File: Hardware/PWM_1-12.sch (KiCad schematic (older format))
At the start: 0 parts

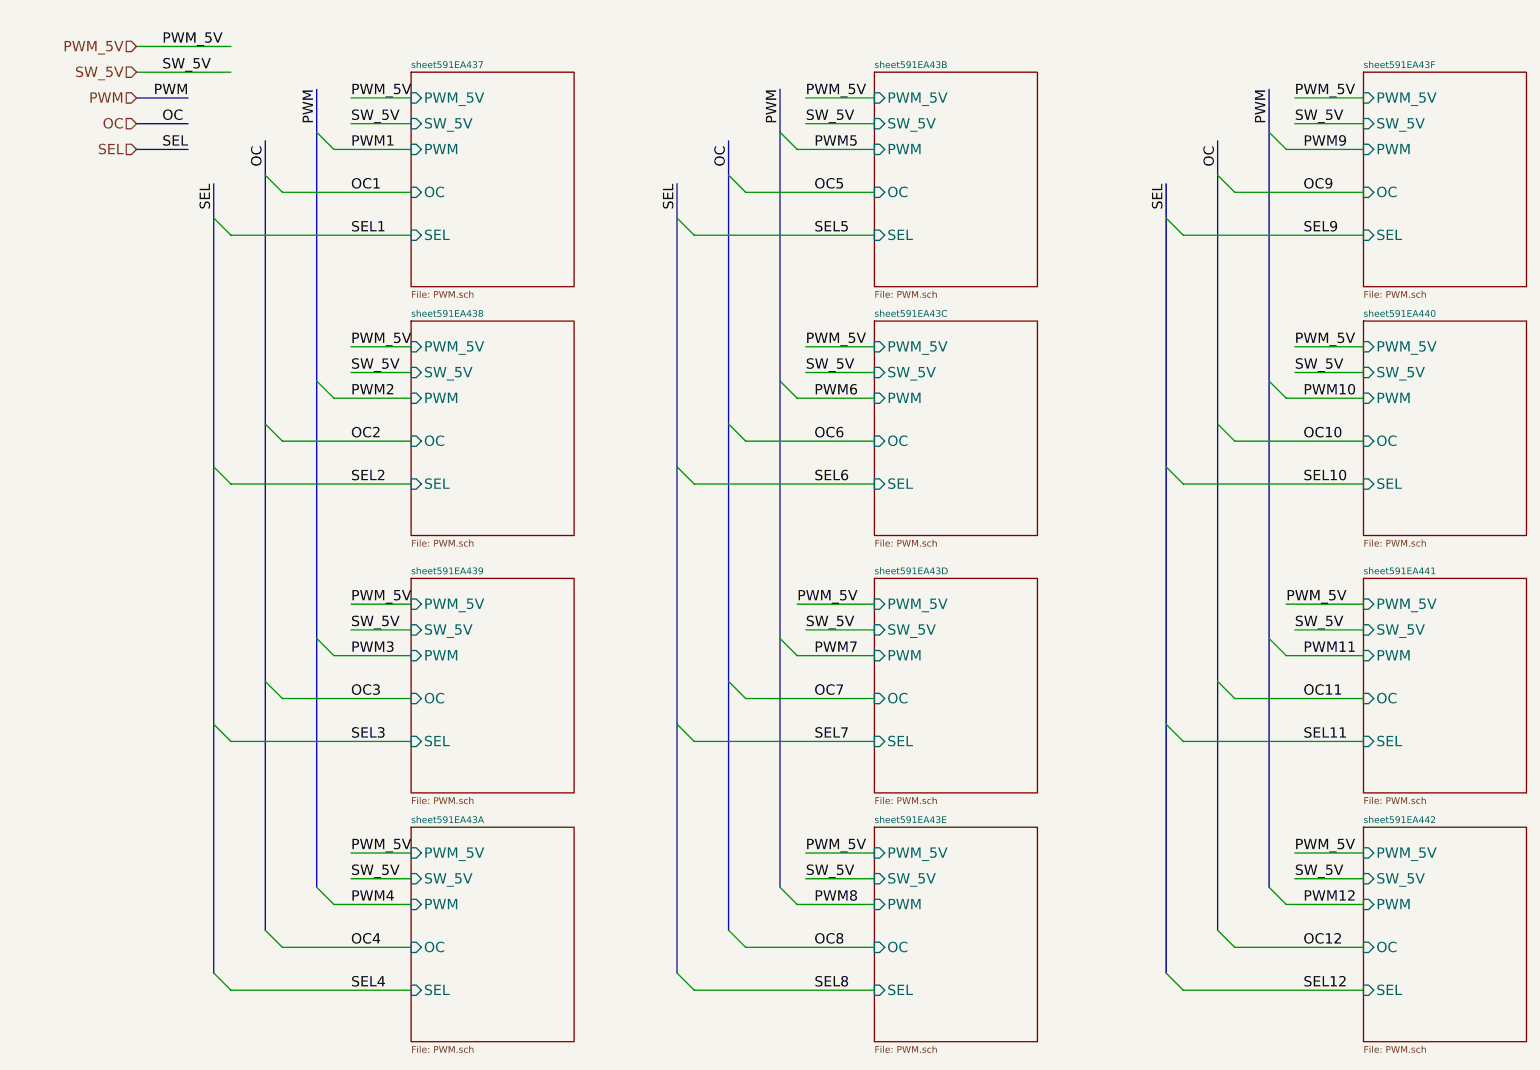
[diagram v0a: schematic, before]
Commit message: Added F7 Circuitry
Added way too much for 1 commit.
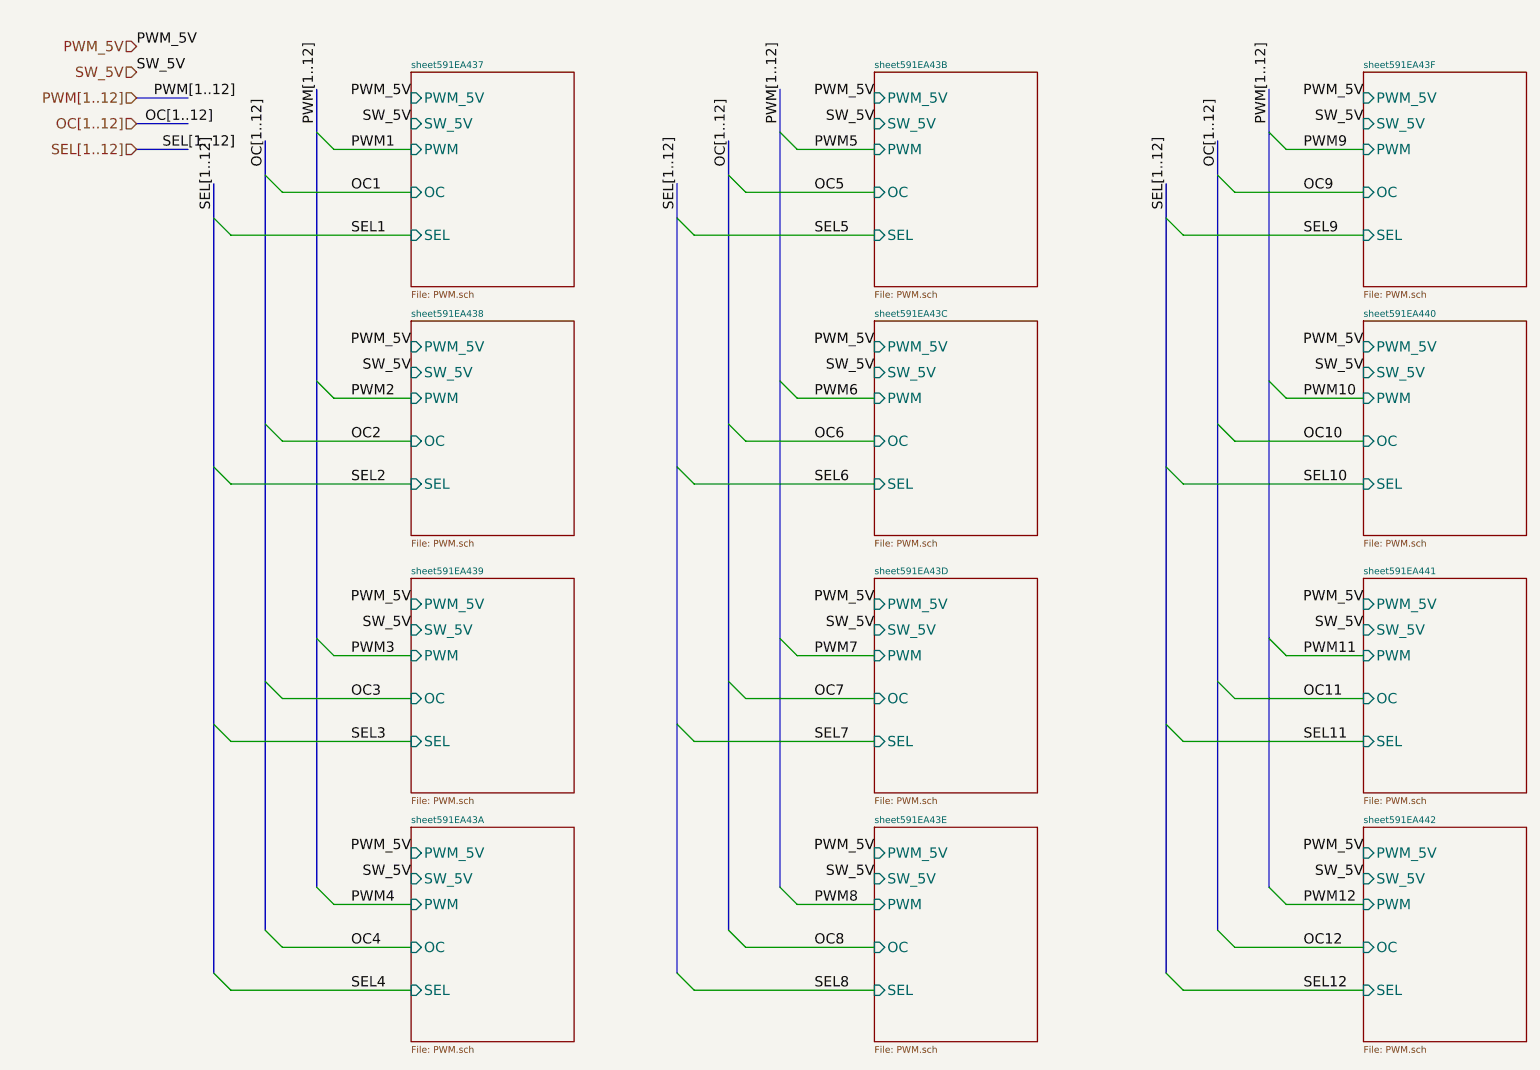
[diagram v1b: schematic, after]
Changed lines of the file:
@@
 LIBS:contrib
 LIBS:valves
+LIBS:ZeroPilot-cache
 EELAYER 25 0
 EELAYER END
 $Descr A4 11693 8268
 encoding utf-8
-Sheet 2 18
+Sheet 2 17
 Title "PWM 1-12"
 Date "2017-05-13"
@@
 PWM4
 Text Label 2150 1100 1    60   ~ 0
-PWM
+PWM[1..12]
 Entry Wire Line
 	1850 5800 1950 5900
@@
 	1850 1400 1950 1500
 Text Label 1850 1350 1    60   ~ 0
-OC
+OC[1..12]
 Entry Wire Line
 	1550 6050 1650 6150
@@
 	1550 1650 1650 1750
 Text Label 1550 1600 1    60   ~ 0
-SEL
+SEL[1..12]
 Text Label 2350 1500 0    60   ~ 0
 OC1
@@
 PWM8
 Text Label 4850 1100 1    60   ~ 0
-PWM
+PWM[1..12]
 Entry Wire Line
 	4550 5800 4650 5900
@@
 	4550 1400 4650 1500
 Text Label 4550 1350 1    60   ~ 0
-OC
+OC[1..12]
 Entry Wire Line
 	4250 6050 4350 6150
@@
 	4250 1650 4350 1750
 Text Label 4250 1600 1    60   ~ 0
-SEL
+SEL[1..12]
 Text Label 5050 1500 0    60   ~ 0
 OC5
@@
 PWM12
 Text Label 7700 1100 1    60   ~ 0
-PWM
+PWM[1..12]
 Entry Wire Line
 	7400 5800 7500 5900
@@
 	7400 1400 7500 1500
 Text Label 7400 1350 1    60   ~ 0
-OC
+OC[1..12]
 Entry Wire Line
 	7100 6050 7200 6150
@@
 	7100 1650 7200 1750
 Text Label 7100 1600 1    60   ~ 0
-SEL
+SEL[1..12]
 Text Label 7900 1500 0    60   ~ 0
 OC9
@@
 Text Label 7900 6150 0    60   ~ 0
 SEL12
-Wire Wire Line
-	2700 950  2350 950
-Wire Wire Line
-	1100 650  1650 650
-Wire Wire Line
-	2350 5350 2700 5350
-Wire Wire Line
-	5400 950  5000 950
-Wire Wire Line
-	5000 5350 5400 5350
-Wire Wire Line
-	5400 3900 4950 3900
-Wire Wire Line
-	5400 2400 5000 2400
-Wire Wire Line
-	8250 950  7850 950
-Wire Wire Line
-	7850 5350 8250 5350
-Wire Wire Line
-	8250 3900 7800 3900
-Wire Wire Line
-	8250 2400 7850 2400
 Wire Bus Line
 	2150 900  2150 5550
@@
 	2250 5650 2700 5650
 Wire Wire Line
-	2700 3900 2350 3900
-Wire Wire Line
 	2250 4200 2700 4200
-Wire Wire Line
-	2700 2400 2350 2400
 Wire Wire Line
 	2700 2700 2250 2700
@@
 	7200 1750 8250 1750
 Text HLabel 1100 1100 0    60   Input ~ 0
-OC
+OC[1..12]
 Text HLabel 1100 950  0    60   Input ~ 0
-PWM
+PWM[1..12]
 Text HLabel 1100 1250 0    60   Input ~ 0
-SEL
+SEL[1..12]
 Text HLabel 1100 650  0    60   Input ~ 0
 PWM_5V
@@
 	1100 1250 1400 1250
 Text Label 1200 950  0    60   ~ 0
-PWM
-Text Label 1250 1100 0    60   ~ 0
-OC
+PWM[1..12]
+Text Label 1150 1100 0    60   ~ 0
+OC[1..12]
 Text Label 1250 1250 0    60   ~ 0
-SEL
-Text Label 2350 950  0    60   ~ 0
-PWM_5V
-Text Label 2350 2400 0    60   ~ 0
-PWM_5V
-Text Label 2350 3900 0    60   ~ 0
-PWM_5V
-Text Label 2350 5350 0    60   ~ 0
-PWM_5V
-Text Label 5000 950  0    60   ~ 0
-PWM_5V
-Text Label 5000 2400 0    60   ~ 0
-PWM_5V
-Text Label 4950 3900 0    60   ~ 0
-PWM_5V
-Text Label 5000 5350 0    60   ~ 0
-PWM_5V
-Text Label 7850 950  0    60   ~ 0
-PWM_5V
-Text Label 7850 2400 0    60   ~ 0
-PWM_5V
-Text Label 7800 3900 0    60   ~ 0
-PWM_5V
-Text Label 7850 5350 0    60   ~ 0
-PWM_5V
-Text Label 1250 650  0    60   ~ 0
-PWM_5V
-Wire Wire Line
-	2700 1100 2350 1100
-Wire Wire Line
-	2350 2550 2700 2550
-Wire Wire Line
-	2350 4050 2700 4050
-Wire Wire Line
-	2700 5500 2350 5500
-Wire Wire Line
-	5000 5500 5400 5500
-Wire Wire Line
-	5000 4050 5400 4050
-Wire Wire Line
-	5000 2550 5400 2550
-Wire Wire Line
-	7850 5500 8250 5500
-Wire Wire Line
-	7850 4050 8250 4050
-Wire Wire Line
-	7850 2550 8250 2550
-Wire Wire Line
-	7850 1100 8250 1100
-Wire Wire Line
-	5000 1100 5400 1100
-Text Label 7850 1100 0    60   ~ 0
-SW_5V
-Text Label 7850 2550 0    60   ~ 0
-SW_5V
-Text Label 7850 4050 0    60   ~ 0
-SW_5V
-Text Label 5000 4050 0    60   ~ 0
-SW_5V
-Text Label 5000 2550 0    60   ~ 0
-SW_5V
-Text Label 5000 1100 0    60   ~ 0
-SW_5V
-Text Label 7850 5500 0    60   ~ 0
-SW_5V
-Text Label 5000 5500 0    60   ~ 0
-SW_5V
-Text Label 2350 5500 0    60   ~ 0
-SW_5V
-Text Label 2350 4050 0    60   ~ 0
-SW_5V
-Text Label 2350 2550 0    60   ~ 0
-SW_5V
-Text Label 2350 1100 0    60   ~ 0
+SEL[1..12]
+Text Label 2700 950  2    60   ~ 0
+PWM_5V
+Text Label 2700 2400 2    60   ~ 0
+PWM_5V
+Text Label 2700 3900 2    60   ~ 0
+PWM_5V
+Text Label 2700 5350 2    60   ~ 0
+PWM_5V
+Text Label 5400 950  2    60   ~ 0
+PWM_5V
+Text Label 5400 2400 2    60   ~ 0
+PWM_5V
+Text Label 5400 3900 2    60   ~ 0
+PWM_5V
+Text Label 5400 5350 2    60   ~ 0
+PWM_5V
+Text Label 8250 950  2    60   ~ 0
+PWM_5V
+Text Label 8250 2400 2    60   ~ 0
+PWM_5V
+Text Label 8250 3900 2    60   ~ 0
+PWM_5V
+Text Label 8250 5350 2    60   ~ 0
+PWM_5V
+Text Label 1100 650  0    60   ~ 0
+PWM_5V
+Text Label 8250 1100 2    60   ~ 0
+SW_5V
+Text Label 8250 2550 2    60   ~ 0
+SW_5V
+Text Label 8250 4050 2    60   ~ 0
+SW_5V
+Text Label 5400 4050 2    60   ~ 0
+SW_5V
+Text Label 5400 2550 2    60   ~ 0
+SW_5V
+Text Label 5400 1100 2    60   ~ 0
+SW_5V
+Text Label 8250 5500 2    60   ~ 0
+SW_5V
+Text Label 5400 5500 2    60   ~ 0
+SW_5V
+Text Label 2700 5500 2    60   ~ 0
+SW_5V
+Text Label 2700 4050 2    60   ~ 0
+SW_5V
+Text Label 2700 2550 2    60   ~ 0
+SW_5V
+Text Label 2700 1100 2    60   ~ 0
 SW_5V
 Text HLabel 1100 800  0    60   Input ~ 0
 SW_5V
-Wire Wire Line
-	1100 800  1650 800
-Text Label 1250 800  0    60   ~ 0
+Text Label 1100 800  0    60   ~ 0
 SW_5V
 $EndSCHEMATC
